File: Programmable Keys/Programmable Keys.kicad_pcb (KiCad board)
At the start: 2 copper layers, 76.2 x 57.1 mm, 20 parts, among them J1 Conn_01x19_Female, J2 Conn_01x19_Male

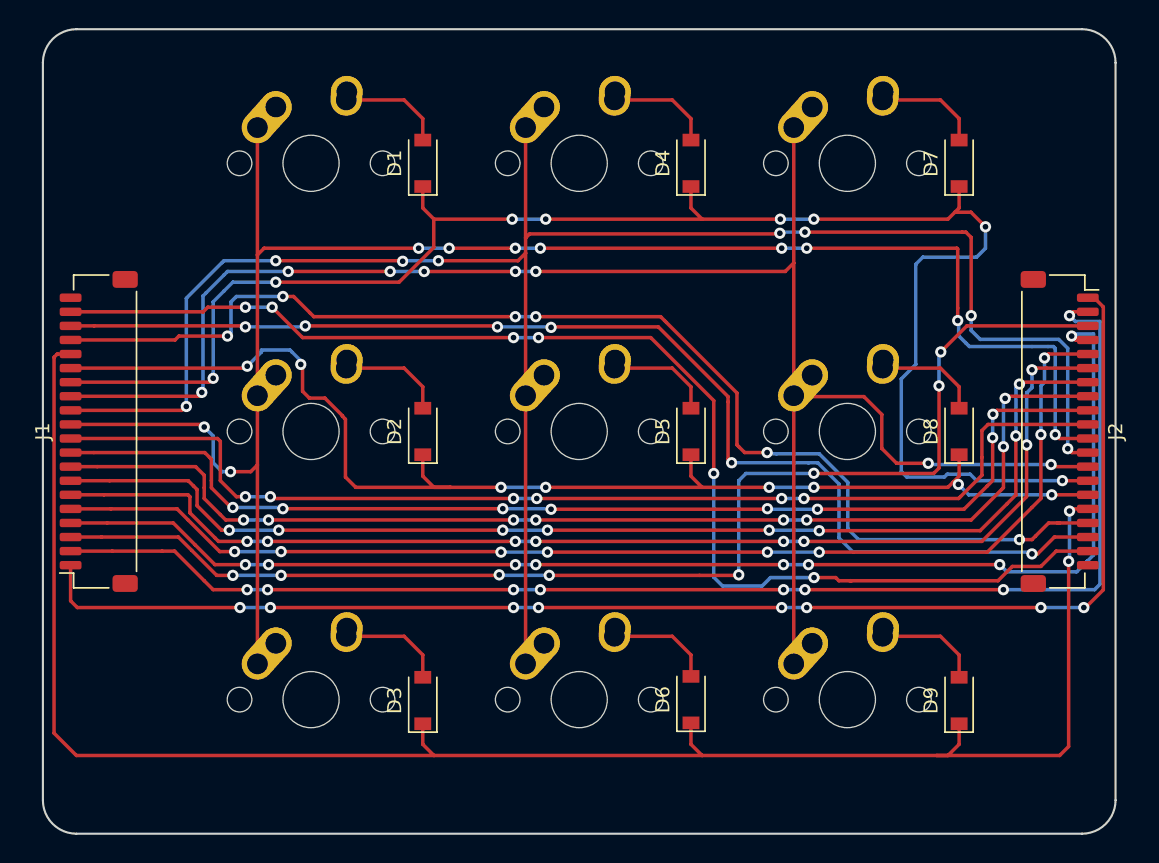
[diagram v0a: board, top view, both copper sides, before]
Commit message: Finished pcb
for now
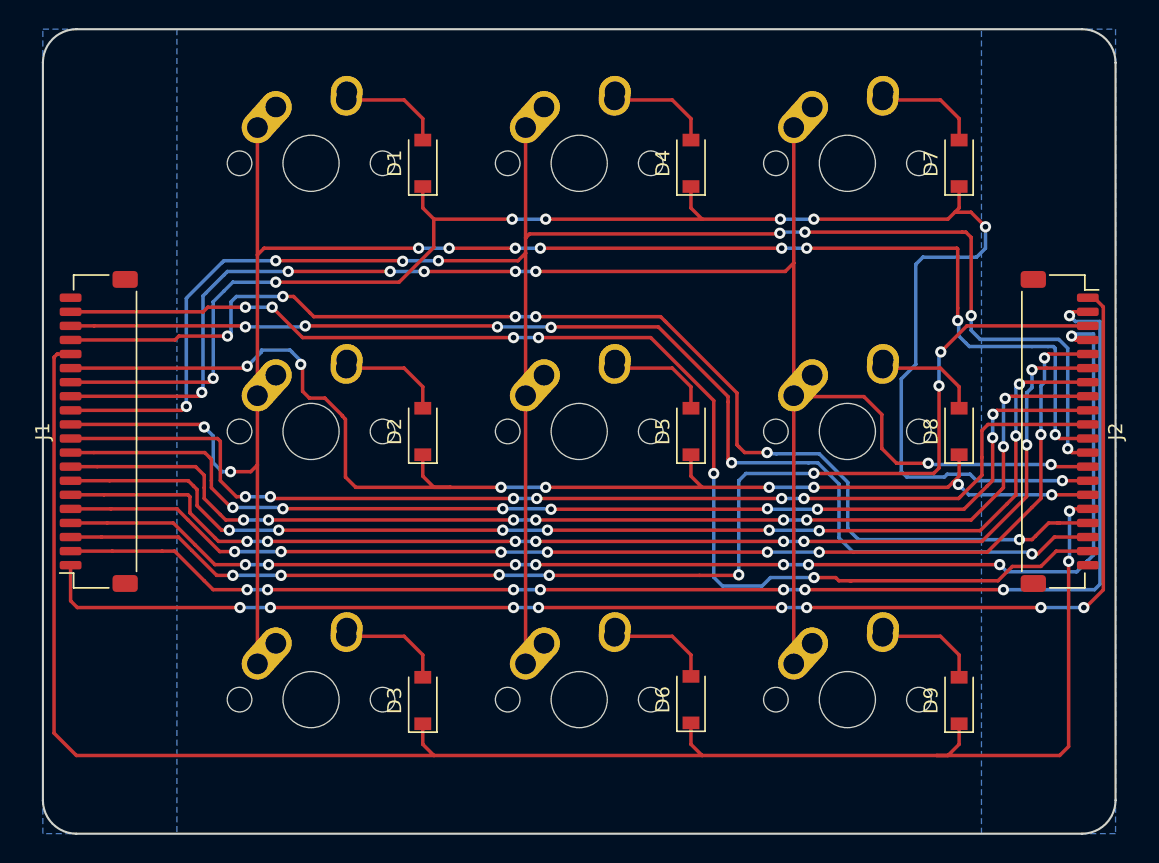
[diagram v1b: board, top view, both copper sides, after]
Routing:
- added copper zone on B.Cu, net GND
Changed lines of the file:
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@@
   (segment (start 202.692 93.472) (end 200.914 93.472) (width 0.25) (layer "B.Cu") (net 28))
   (segment (start 222.377 93.472) (end 219.329 93.472) (width 0.25) (layer "B.Cu") (net 28))
+  (zone (net 16) (net_name "GND") (layer "B.Cu") (hatch edge 0.508)
+    (connect_pads (clearance 0.508))
+    (min_thickness 0.254) (filled_areas_thickness no)
+    (fill yes (thermal_gap 0.508) (thermal_bridge_width 0.508))
+    (polygon
+      (pts
+        (xy 157.95625 109.5375)
+        (xy 148.43125 109.5375)
+        (xy 148.43125 52.3875)
+        (xy 157.95625 52.3875)
+      )
+    )
+  )
+  (zone (net 16) (net_name "GND") (layer "B.Cu") (hatch edge 0.508)
+    (connect_pads (clearance 0.508))
+    (min_thickness 0.254) (filled_areas_thickness no)
+    (fill yes (thermal_gap 0.508) (thermal_bridge_width 0.508))
+    (polygon
+      (pts
+        (xy 224.63125 109.5375)
+        (xy 215.10625 109.5375)
+        (xy 215.10625 52.3875)
+        (xy 224.63125 52.3875)
+      )
+    )
+  )
 )
